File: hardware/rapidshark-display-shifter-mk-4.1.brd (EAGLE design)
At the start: 20.3 x 20.3 mm, 12 parts, among them U1 ADAFRUIT_FEATHER_SHIELDSMALLH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, U2 SPARKFUN_MICROVIEWSMALLHOLES

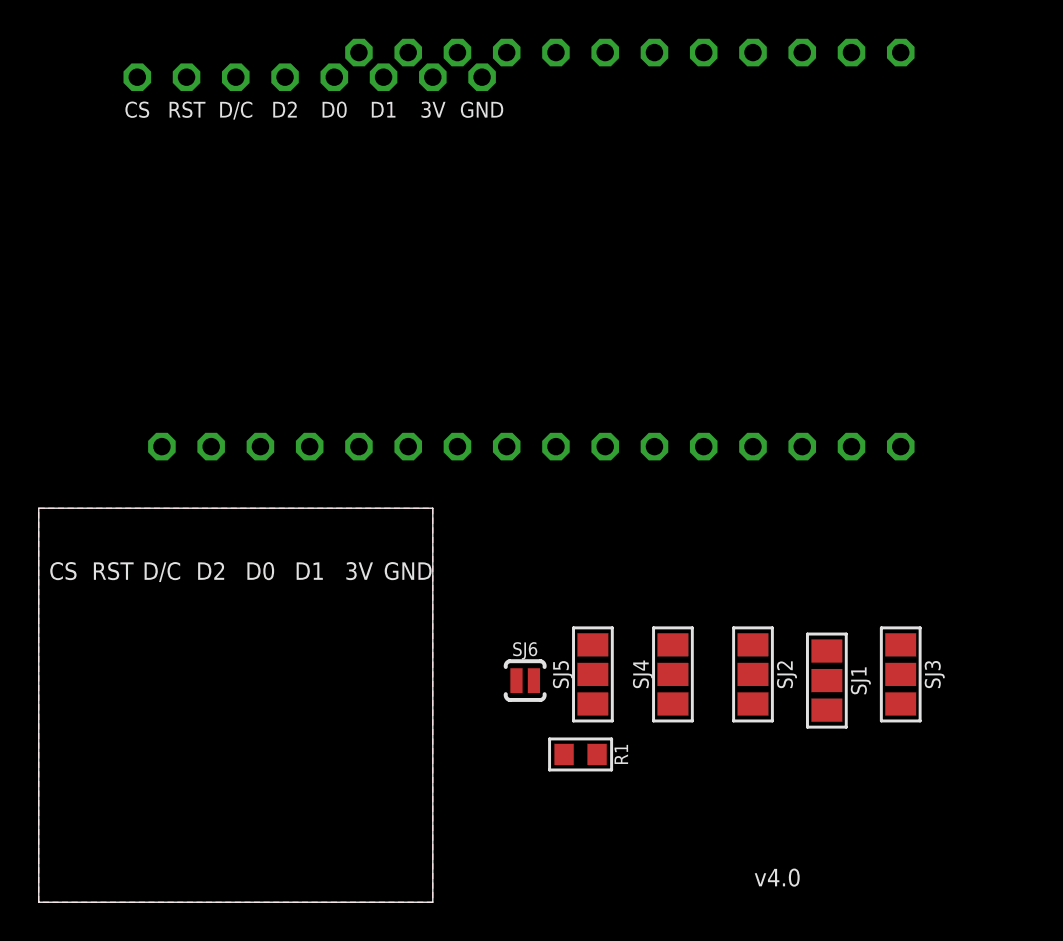
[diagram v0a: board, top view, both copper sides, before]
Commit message: adding these to commit to log before shifting to another repo
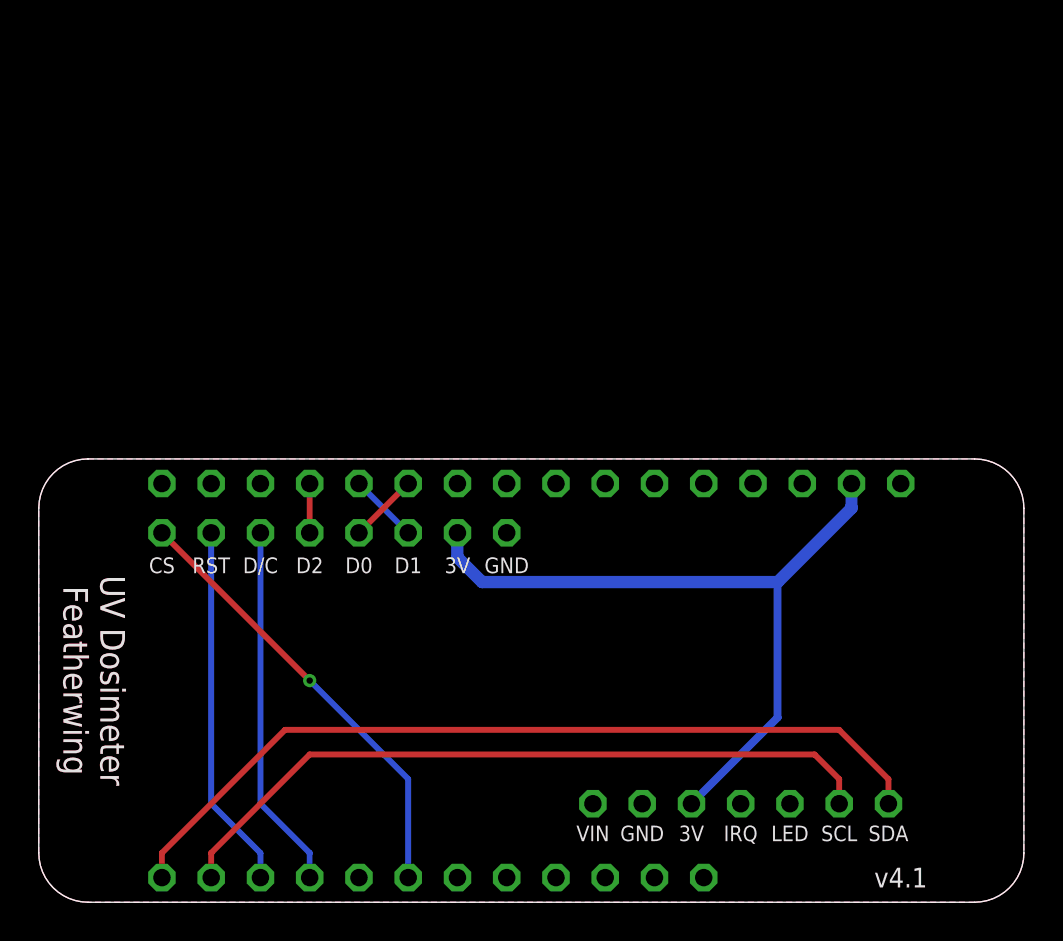
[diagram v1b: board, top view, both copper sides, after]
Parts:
- removed R1: 10K, a_parts:R0603
- removed SJ1, SJ2, SJ3, SJ4: I2C SPI, a_parts:PAD-JUMPER-3-NO_YES_SILK_FULL_BOX
- removed SJ5: 3C 3D, a_parts:PAD-JUMPER-3-NO_YES_SILK_FULL_BOX
- removed SJ6: JUMPER-PAD-2-NOYES_SILK, a_parts:PAD-JUMPER-2-NO_YES_SILK
- added U3: ADAFRUIT-SI1145-BREAKOUTSMALLHOLES, a_parts:ADAFRUIT-SI1145-BREAKOUT-LESSSILK-SMALLHOLES
- moved U2 23.5 mm to (15.2, 10.2)
- moved U1 22.2 mm to (25.4, 11.4), turned to 180 degrees
- moved U$1 19.1 mm to (25.4, 12.7)
- moved U$3 8.28 mm to (45.1, 1.91)
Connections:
- removed net D/C: U2.D/C
- removed net MISO: SJ3.3, U1.MISO
- removed net MOSI: SJ1.3, U1.MOSI
- removed net N$1: R1.1, SJ5.1
- removed net N$2: SJ4.1, SJ5.2
- removed net SCK: SJ2.3, U1.SCK
- removed net SHIELD_CS: SJ6.2, U1.10
- removed net SHIELD_D/C: SJ4.3, U1.6
- new net DATA/CMD: U1.6, U2.D/C
- net 3.3V: now also U3.3V3_OUT; no longer R1.2
- net D0: now also U1.SCK; no longer SJ2.2
- net D1: now also U1.MOSI
- net D2: now also U1.MISO
- net DISP_CS: now also U1.10; no longer SJ6.1
- net GND: now also U3.GND; no longer SJ5.3
- net SCL: now also U3.SCL; no longer SJ2.1
- net SDA: now also U3.SDA; no longer SJ1.1
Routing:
- net SDA: track 0.00 -> 43.7 mm
- net 3.3V: track 0.00 -> 38.2 mm
- net SCL: track 0.00 -> 37.6 mm
- net DISP_CS: track 0.00 -> 23.0 mm, vias 0 -> 1
- net DISP_RST: track 0.00 -> 18.8 mm
- net DATA/CMD: track 0.00 -> 18.8 mm
- net D1: track 0.00 -> 3.59 mm
- net D0: track 0.00 -> 3.59 mm
- net D2: track 0.00 -> 2.54 mm
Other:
- board size 20.3 x 20.3 mm -> 50.8 x 22.9 mm
- board text added: "UV Dosimeter Featherwing"
- board text removed: "3V"
- board text removed: "CS"
- board text removed: "D/C"
- board text removed: "D0"
- board text removed: "D1"
- board text removed: "D2"
- board text removed: "GND"
- board text removed: "RST"
